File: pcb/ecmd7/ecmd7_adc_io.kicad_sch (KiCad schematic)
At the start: 80 parts, among them U10 FIN1002M5X, U11 FIN1002M5X, U12 FIN1002M5X, U13 ADM3490ExR, U15 74LVC1G139, U16 MB85RS1MT, U17 TMP122AIDBVR, U2 MCP33151-05T-E/MN, U4 MCP33151-05T-E/MN, U5 MCP33151-05T-E/MN, U7 MCP33151-05T-E/MN

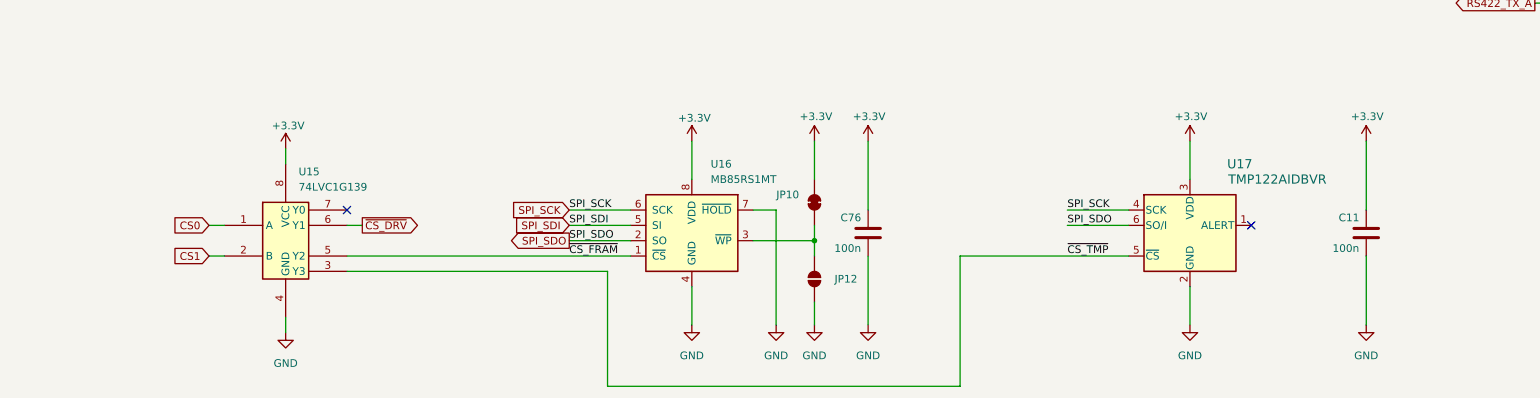
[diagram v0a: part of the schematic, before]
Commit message: Final layout
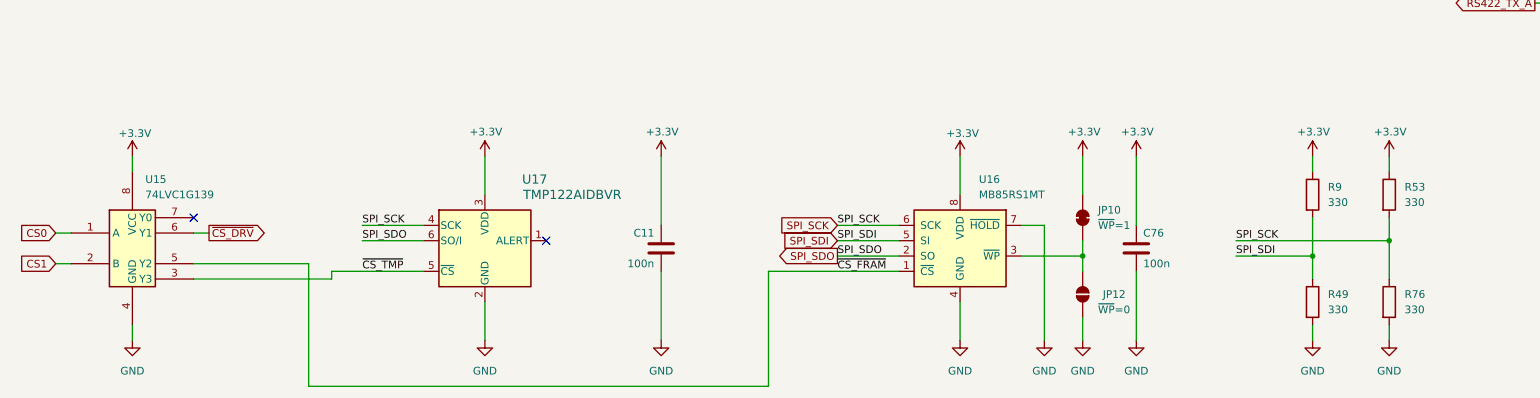
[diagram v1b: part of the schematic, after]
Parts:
- added R49, R53, R76, R9: 330, Resistor_SMD:R_0805_2012Metric, symbol Device:R
- JP10: value SolderJumper_2_Bridged -> ~{WP}=1
- JP12: value SolderJumper_2_Open -> ~{WP}=0
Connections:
- net +3.3V: now also R53.1, R9.1
- net GND: now also R49.2, R76.2
- net SPI_SCK: now also R53.2, R76.1
- net SPI_SDI: now also R49.1, R9.2
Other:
- moved on the sheet: C11, C76, JP10, JP12, U15, U16, U17
